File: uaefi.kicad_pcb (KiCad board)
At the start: 4 copper layers, 133.2 x 100 mm, 142 parts, among them J23 2-6447232-3, J25 2-6447232-3, J6 Conn_01x06, J7 Conn_01x05_Male, J8 USB_B_Mini, J9 USB_C, M1 Module-power_12and5V-0.3, M2 Module-knock-0.2, M3 Module-vr-discrete-0.5, M4 Module-vr-max9924-0.1, M5 Module-wbo-0.5, M6 Module:mega-mcu100/0.3, M7 Module-can-0.1, P1 Pad, P15 Pad, P16 Pad, P17 Pad, P18 Pad, P2 Pad, P3 Pad, P4 Pad, P5 Pad, P6 Pad, P7 Pad, P8 Pad, Q10 ISL9V3040D3ST, Q11 ISL9V3040D3ST, Q12 ISL9V3040D3ST, Q7 ISL9V3040D3ST, Q8 ISL9V3040D3ST, Q9 ISL9V3040D3ST, U1 TLE9201SG, U10 VNLD5160TR-E, U11 VNLD5160TR-E, U2 TLE9201SG, U3 MPX4/MPXH6400_MAP, U4 MAX31855KASA, U5 JDY-33, U6 VNLD5160TR-E, U7 VNLD5160TR-E, U8 VNLD5160TR-E, U9 VNLD5160TR-E

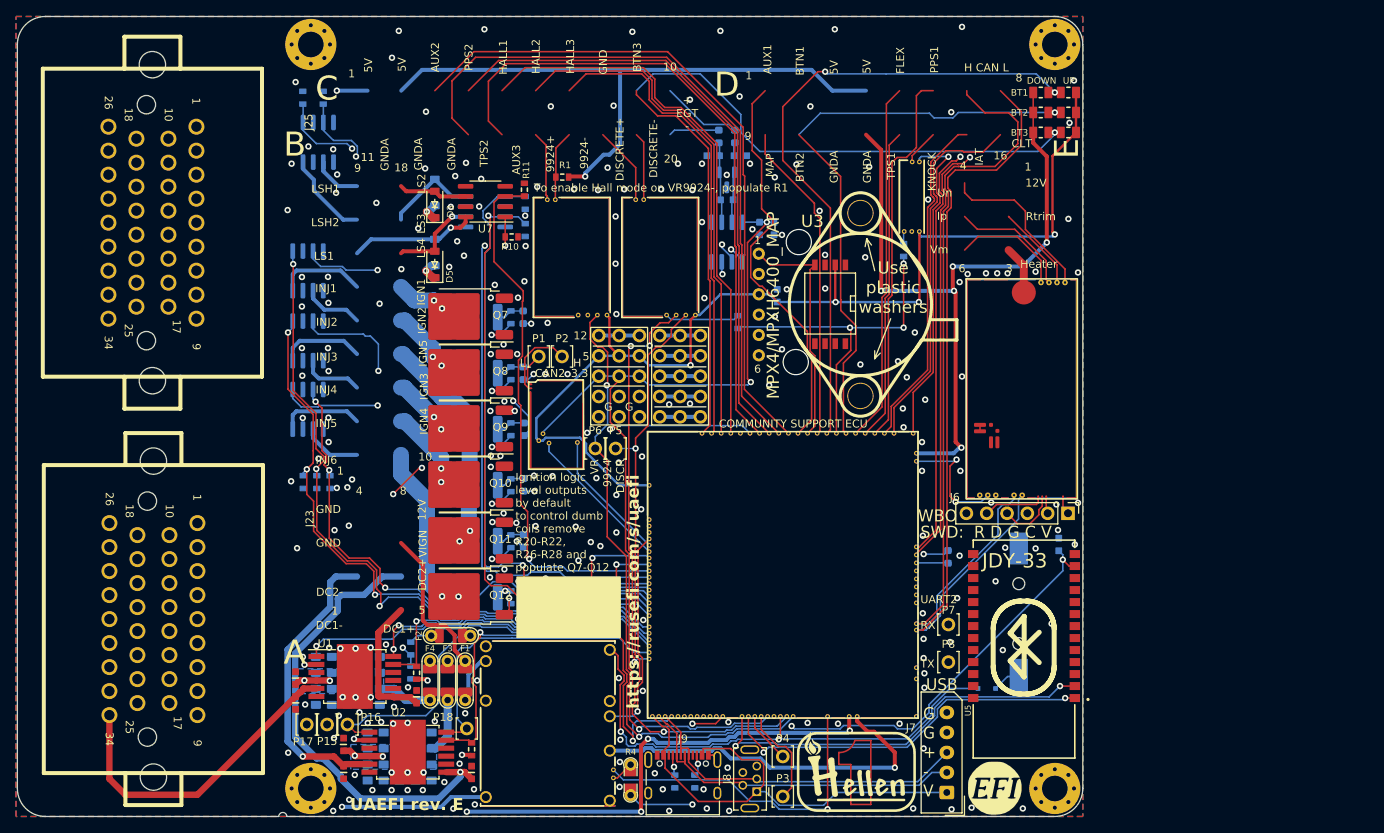
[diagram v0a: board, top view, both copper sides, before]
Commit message: mkn
mnj
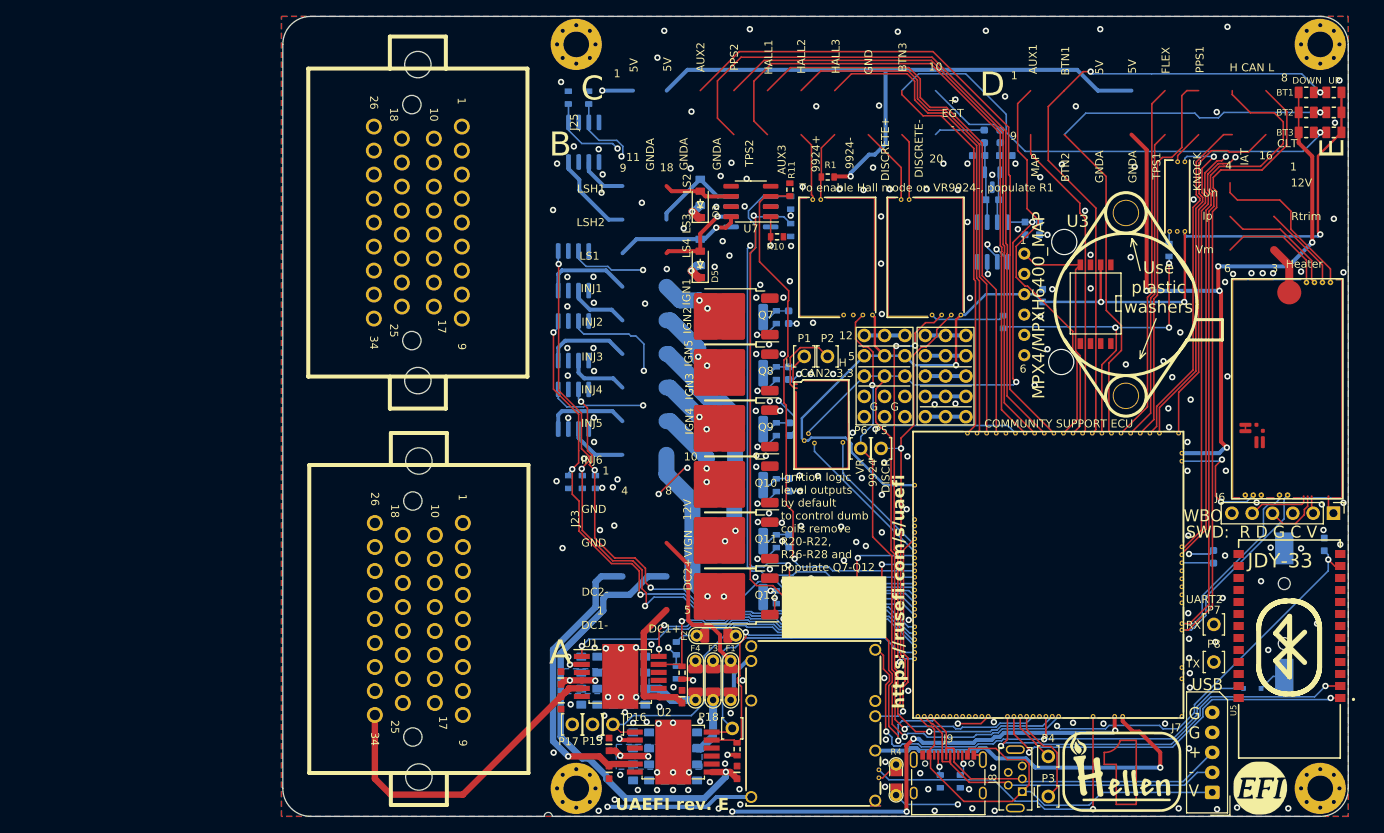
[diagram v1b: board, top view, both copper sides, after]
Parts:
- moved BT1 33.2 mm to (175.2, 134.5)
- moved C13 33.2 mm to (99.9, 145.0)
- moved C16 33.2 mm to (97.8, 150.5)
- moved C17 33.2 mm to (99.8, 150.5)
- moved C18 33.2 mm to (101.8, 150.5)
- moved C21 33.2 mm to (97.8, 154.5)
- moved C22 33.2 mm to (99.8, 154.5)
- moved C23 33.2 mm to (101.8, 154.5)
- moved C26 33.2 mm to (106.8, 154.5)
- moved C29 33.2 mm to (138.7, 82.9)
- moved C30 33.2 mm to (140.4, 77.4)
- moved C31 33.2 mm to (142.8, 86.5)
- moved C33 33.2 mm to (180.2, 126.0)
- moved D1 33.2 mm to (171.2, 144.0)
- moved D8 33.2 mm to (138.7, 80.4)
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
